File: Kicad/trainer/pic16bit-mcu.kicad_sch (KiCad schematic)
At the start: 25 parts, among them K201 MCU 1, K202 MCU 2, K203 ICSP, K204 VIN, K205 VIN, K206 VDD, K207 GND, K208 VDD, K209 GND, K210 HARWIN-254-F-1X10-VERTICAL, U201 PIC24/dsPIC33, X201 XTAL-DIL08

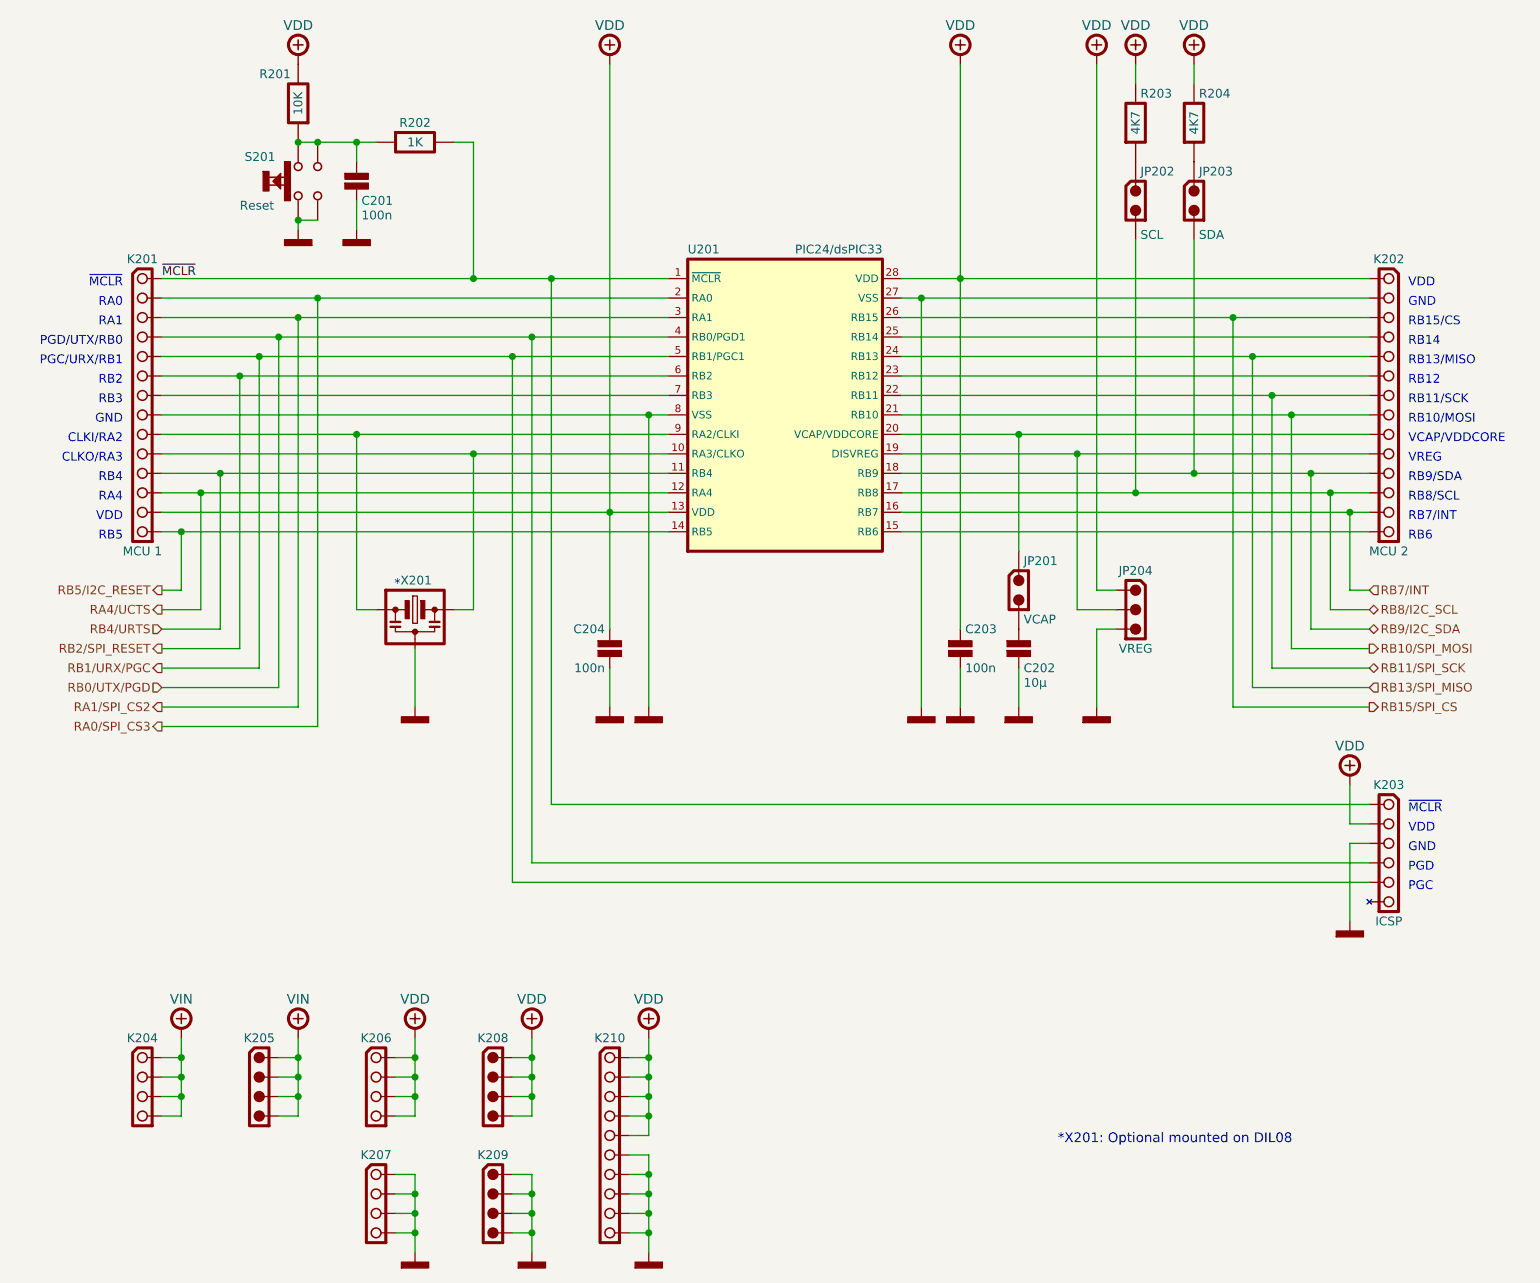
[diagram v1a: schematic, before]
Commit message: Up
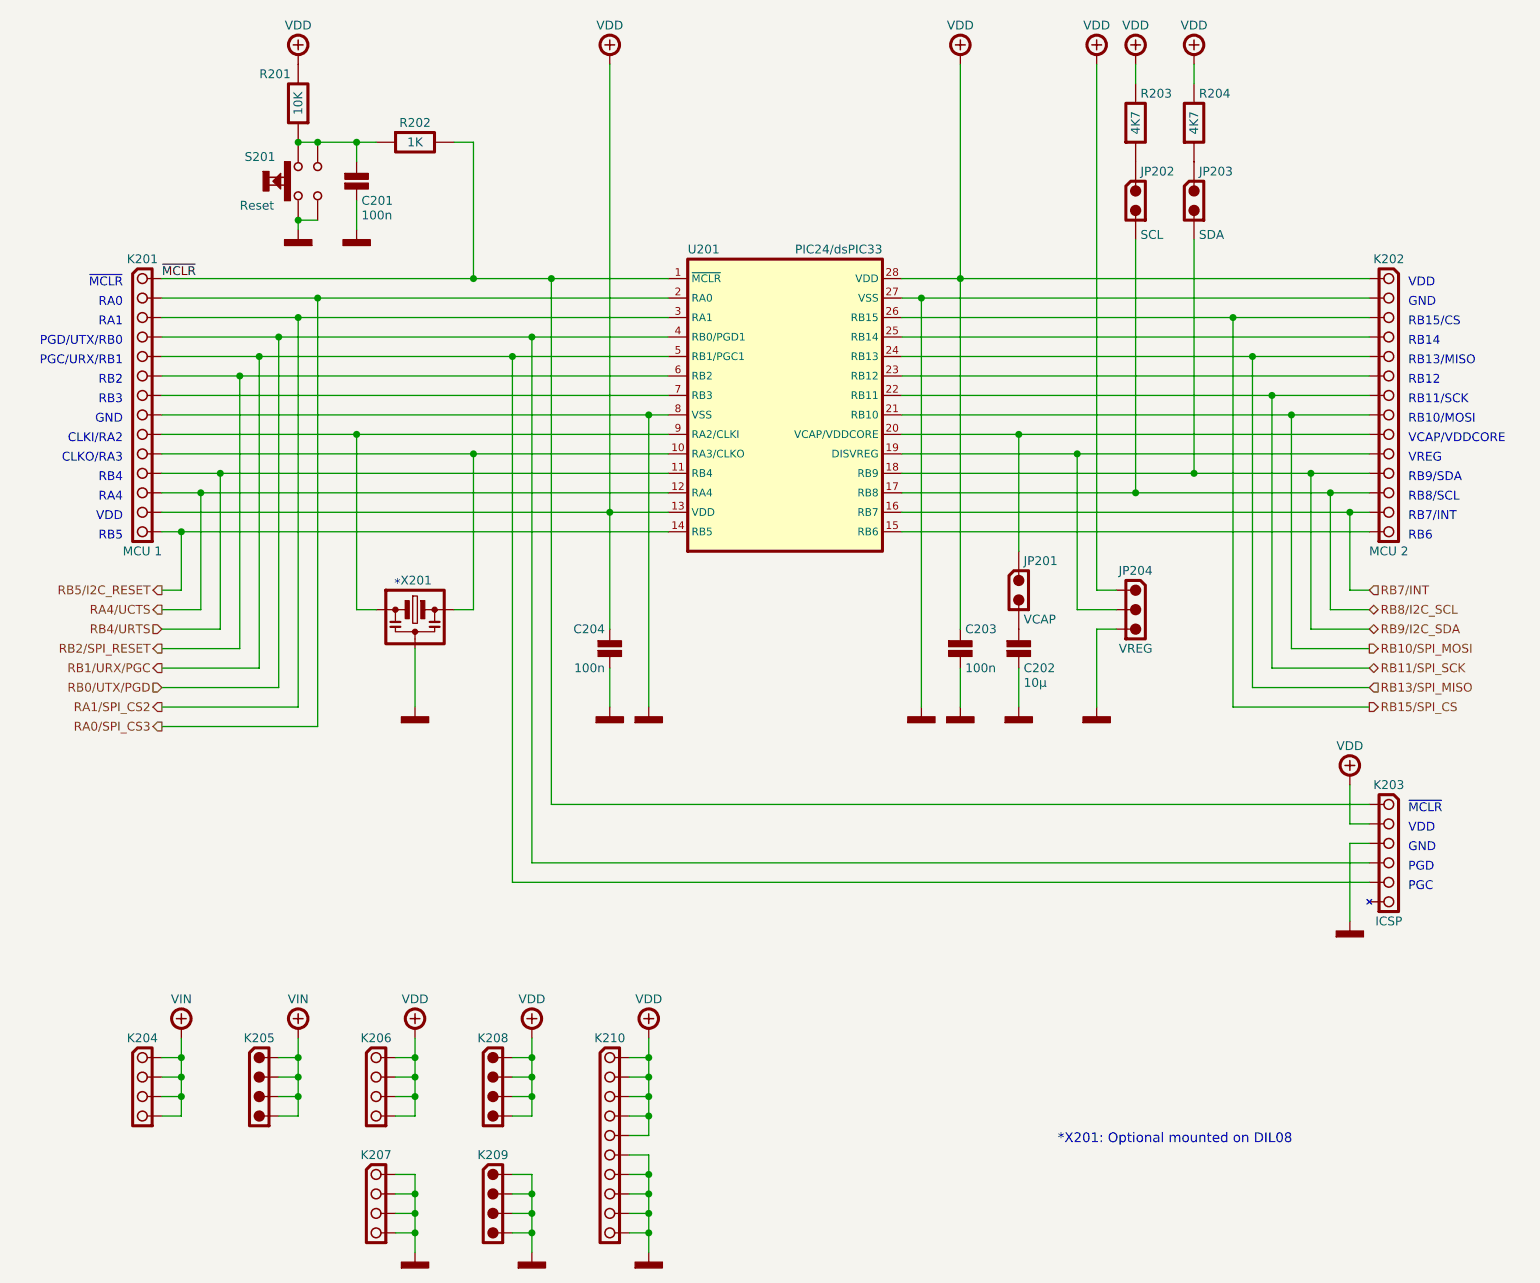
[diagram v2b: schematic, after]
